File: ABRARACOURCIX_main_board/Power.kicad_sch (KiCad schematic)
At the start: 14 parts, among them J2 XT60PW-M, J3 XT60PW-M, Q2 NTR4101PT1G, U3 AZ1117CH-3.3TRG1, U4 LT1529CQ-5_PBF

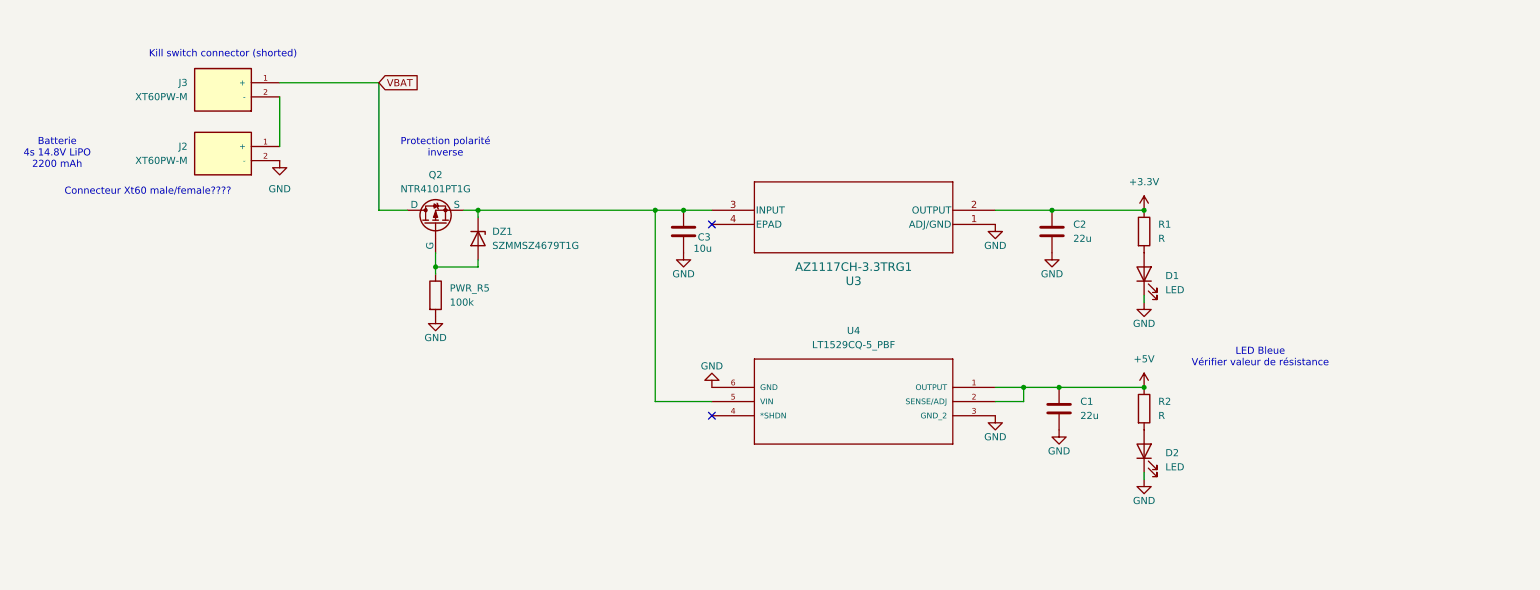
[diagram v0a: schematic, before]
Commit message: Reprise de contrôle
Schematics terminés
Reste à associer des composantes et vérification
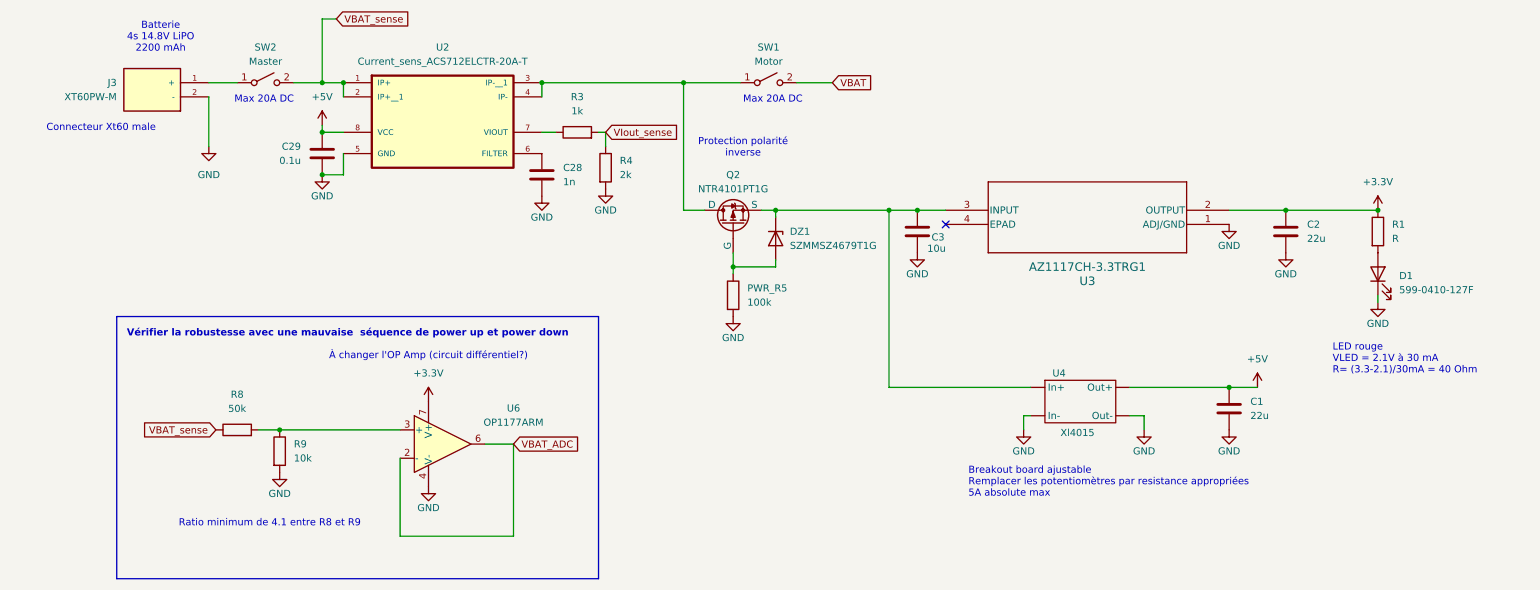
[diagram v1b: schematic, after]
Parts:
- removed D2: LED, symbol Device:LED
- removed J2: XT60PW-M, XT60PW-M:AMASS_XT60PW-M, symbol GAUL_ABRARACOURCIX:XT60PW-M
- removed R2: R, symbol Device:R
- removed U4: LT1529CQ-5_PBF, LT1529CQ-5_PBF:DDPAK-5_Q, symbol GAUL_ABRARACOURCIX:LT1529CQ-5_PBF
- added C28: 1n, symbol Device:C
- added C29: 0.1u, symbol Device:C
- added R3: 1k, symbol Device:R
- added R4: 2k, symbol Device:R
- added R8: 50k, symbol Device:R
- added R9: 10k, symbol Device:R
- added SW1: Motor, symbol Switch:SW_SPST
- added SW2: Master, symbol Switch:SW_SPST
- added U2: Current_sens_ACS712ELCTR-20A-T, ACS712ELCTR-20A-T:SOIC127P600X175-8N, symbol GAUL_ABRARACOURCIX:Current_sens_ACS712ELCTR-20A-T
- added U4: Xl4015, symbol GAUL_ABRARACOURCIX:Buck_Xl4015_breakout
- added U6: OP1177ARM, Package_SO:MSOP-8_3x3mm_P0.65mm, symbol Amplifier_Operational:OP1177ARM
- D1: value LED -> 599-0410-127F; Digikey (none) -> https://www.digikey.ca/en/products/detail/dialight/599-0410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
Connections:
- net +3.3V: now also U6.7 (V+)
- net +5V: now also C29.1, U2.8 (VCC), U4. (Out-)
- net GND: now also J3.2 (-), C28.2, C29.2, R4.2, R9.2, U2.5 (GND), U4. (Out-), U6.4 (V-)
- net VBAT: now also SW1.2 (B); no longer J3.1 (+), Q2.1 (D)
- net at C3.1, DZ1.1 (K), Q2.3 (S)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: now also U4. (Out-)
- new net: R8.2, R9.1, U6.3 (+)
- new net: J3.1 (+), SW2.1 (A)
- new net: R3.1, U2.7 (VIOUT)
- new net: Q2.1 (D), SW1.1 (A), U2.3 (IP-__1), U2.4 (IP-)
- new net: C28.1, U2.6 (FILTER)
- new net VBAT_ADC: U6.2 (-), U6.6
- new net VBAT_sense: R8.1, SW2.2 (B), U2.1 (IP+), U2.2 (IP+__1)
- new net VIout_sense: R3.2, R4.1
- no-connect marks 2 -> 1
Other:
- note added: "Breakout board ajustable Remplacer les potentiomètres par resistance appropriées 5A absolute max"
- note added: "Connecteur Xt60 male"
- note added: "LED rouge VLED = 2.1V à 30 mA R= (3.3-2.1)/30mA = 40 Ohm"
- note added: "Max 20A DC"
- note added: "Ratio minimum de 4.1 entre R8 et R9"
- note added: "Vérifier la robustesse avec une mauvaise séquence de power up et power down"
- note added: "À changer l'OP Amp (circuit différentiel?)"
- note removed: "Connecteur Xt60 male/female????"
- note removed: "Kill switch connector (shorted)"
- note removed: "LED Bleue Vérifier valeur de résistance"
- moved on the sheet: C1, C2, C3, D1, DZ1, J3, PWR_R5, Q2, R1, U3
